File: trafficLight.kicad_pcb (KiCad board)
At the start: 2 copper layers, 11 parts, among them J1 Conn_01x04

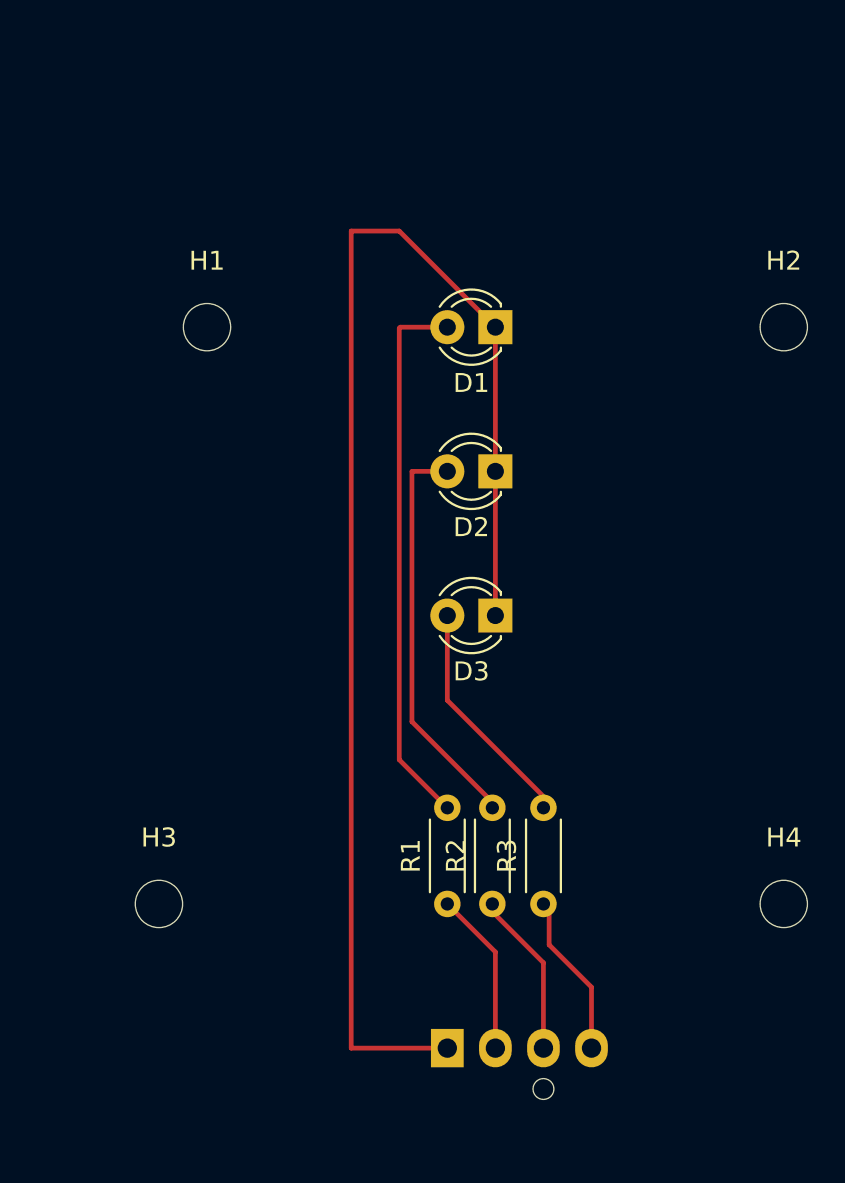
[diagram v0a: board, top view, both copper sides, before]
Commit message: Recent modicifation of layout
i	deleted:    trafficLight-backups/trafficLight-2022-02-05_192826.zip
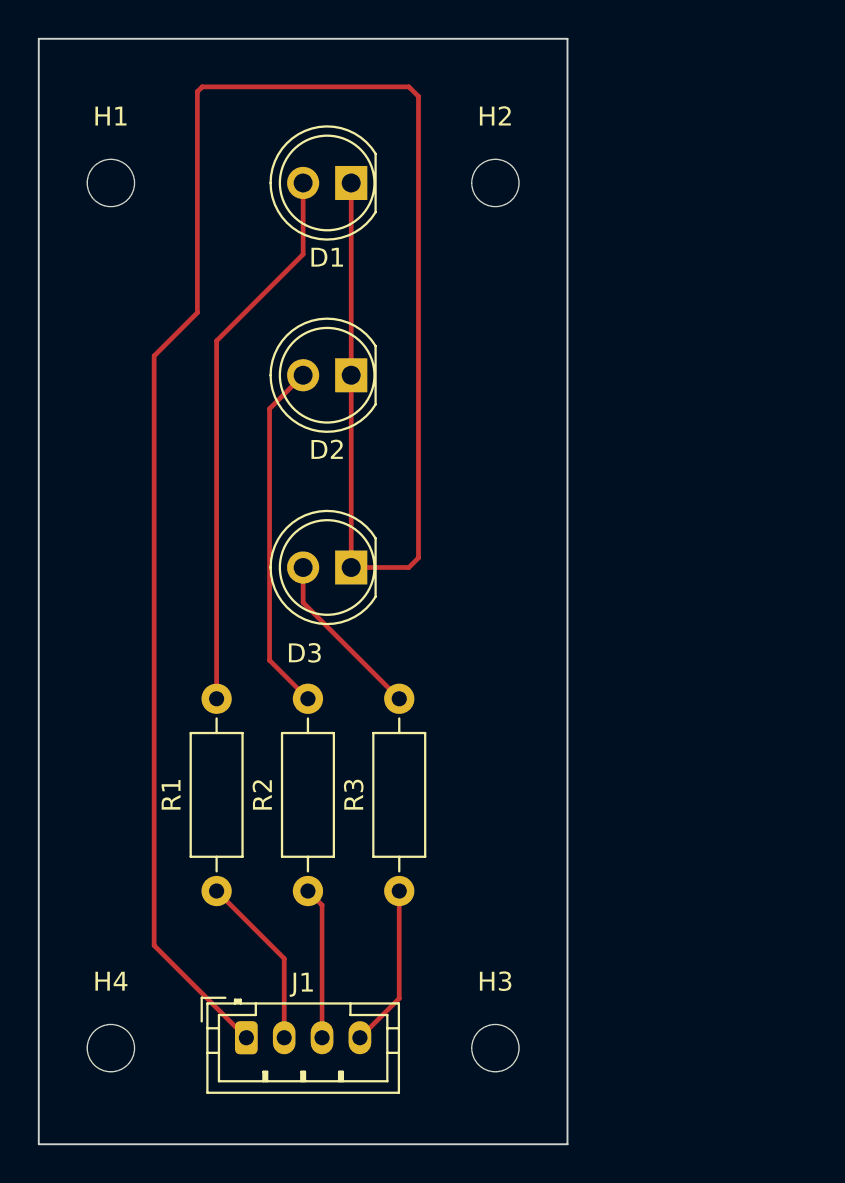
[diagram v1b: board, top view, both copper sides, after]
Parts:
- D1, D2, D3: footprint LED_THT:LED_D3.0mm -> LED_THT:LED_D5.0mm
- J1: footprint Connector:FanPinHeader_1x04_P2.54mm_Vertical -> Connector_JST:JST_PH_B4B-PH-K_1x04_P2.00mm_Vertical; moved to F.Cu
- R1, R2, R3: footprint Resistor_THT:R_Axial_DIN0204_L3.6mm_D1.6mm_P5.08mm_Horizontal -> Resistor_THT:R_Axial_DIN0207_L6.3mm_D2.5mm_P10.16mm_Horizontal
- moved H4 36.4 mm to (116.8, 124.5)
- moved H3 19.3 mm to (137.2, 124.5)
- moved H2 17.0 mm to (137.2, 78.7)
- moved R1 12.2 mm to (122.4, 116.2)
- moved D1 10.8 mm to (129.5, 78.7)
- moved J1 10.6 mm to (124.0, 123.9)
- moved R2 9.77 mm to (127.3, 116.2)
- moved D2 9.16 mm to (129.5, 88.9)
- moved H1 9.16 mm to (116.8, 78.7)
- moved D3 8.03 mm to (129.5, 99.1)
- moved R3 7.65 mm to (132.1, 116.2)
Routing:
- net Net-(D1-Pad1): track 73.2 -> 113.4 mm
- net Net-(D3-Pad2): track 12.1 -> 9.04 mm
- net Net-(D2-Pad2): track 21.5 -> 18.7 mm
- net Net-(J1-Pad3): track 9.04 -> 8.06 mm
- net Net-(J1-Pad2): track 8.67 -> 9.23 mm
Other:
- board outline added: 27.9 x 58.4 mm
